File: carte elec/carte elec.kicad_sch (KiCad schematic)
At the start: 47 parts, among them J1 SD_Card_Device, J2 Barrel_Jack_Switch, U1 ESP32-S3-UNO, U2 R-78E5.0-1.0

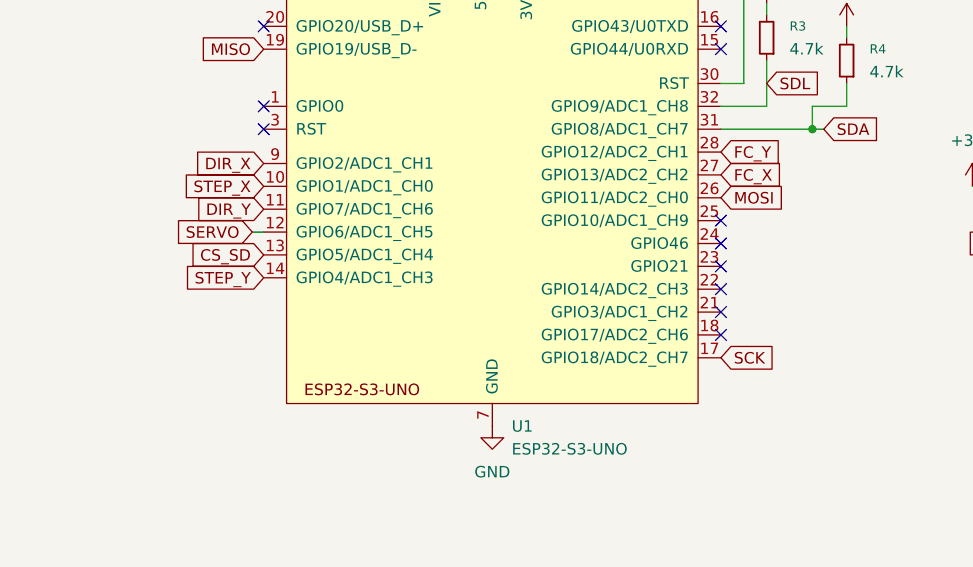
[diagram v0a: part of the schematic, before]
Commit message: Add files via upload
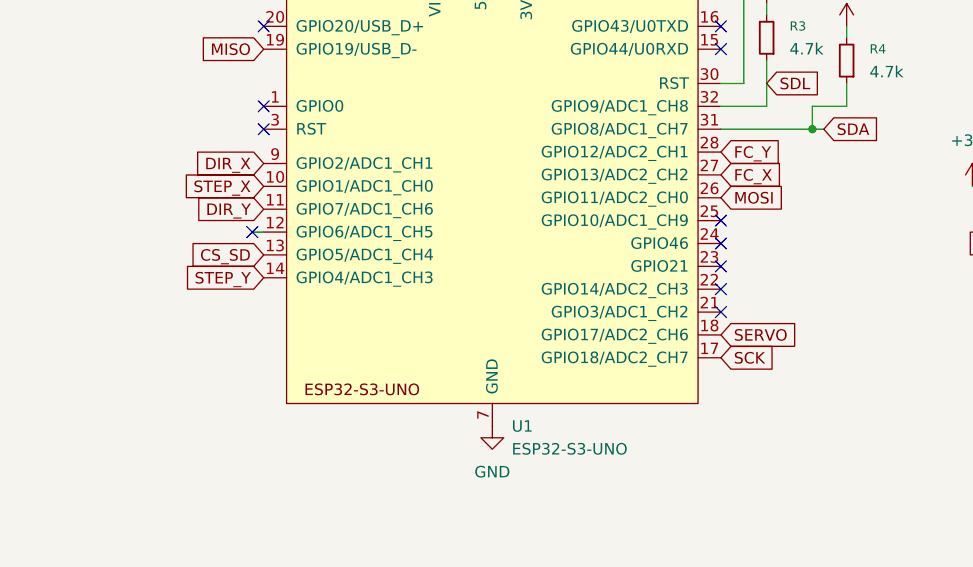
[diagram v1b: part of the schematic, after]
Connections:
- net SERVO: now also U1.18 (GPIO17/ADC2_CH6); no longer U1.12 (GPIO6/ADC1_CH5)
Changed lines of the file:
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@@
+	)
+	(no_connect
+		(at 143.51 129.54)
 	)
 	(no_connect
@@
 	(no_connect
 		(at 248.92 26.67)
-	)
-	(no_connect
-		(at 195.58 140.97)
 	)
 	(no_connect
@@
 		)
 	)
+	(global_label "SERVO"
+		(shape input)
+		(at 195.58 140.97 0)
+		(fields_autoplaced yes)
+		(effects
+			(font
+				(size 1.27 1.27)
+			)
+			(justify left)
+		)
+		(property "Intersheetrefs" "${INTERSHEET_REFS}"
+			(at 204.6128 140.97 0)
+			(effects
+				(font
+					(size 1.27 1.27)
+				)
+				(justify left)
+				(hide yes)
+			)
+		)
+	)
 	(global_label "CS_SD"
 		(shape input)
@@
 			(effects
 				(font
-					(size 1.27 1.27)
-				)
-				(justify right)
-				(hide yes)
-			)
-		)
-	)
-	(global_label "SERVO"
-		(shape input)
-		(at 143.51 129.54 180)
-		(fields_autoplaced yes)
-		(effects
-			(font
-				(size 1.27 1.27)
-			)
-			(justify right)
-		)
-		(property "Intersheetrefs" "${INTERSHEET_REFS}"
-			(at 134.4772 129.54 0)
-			(effects
-				(font

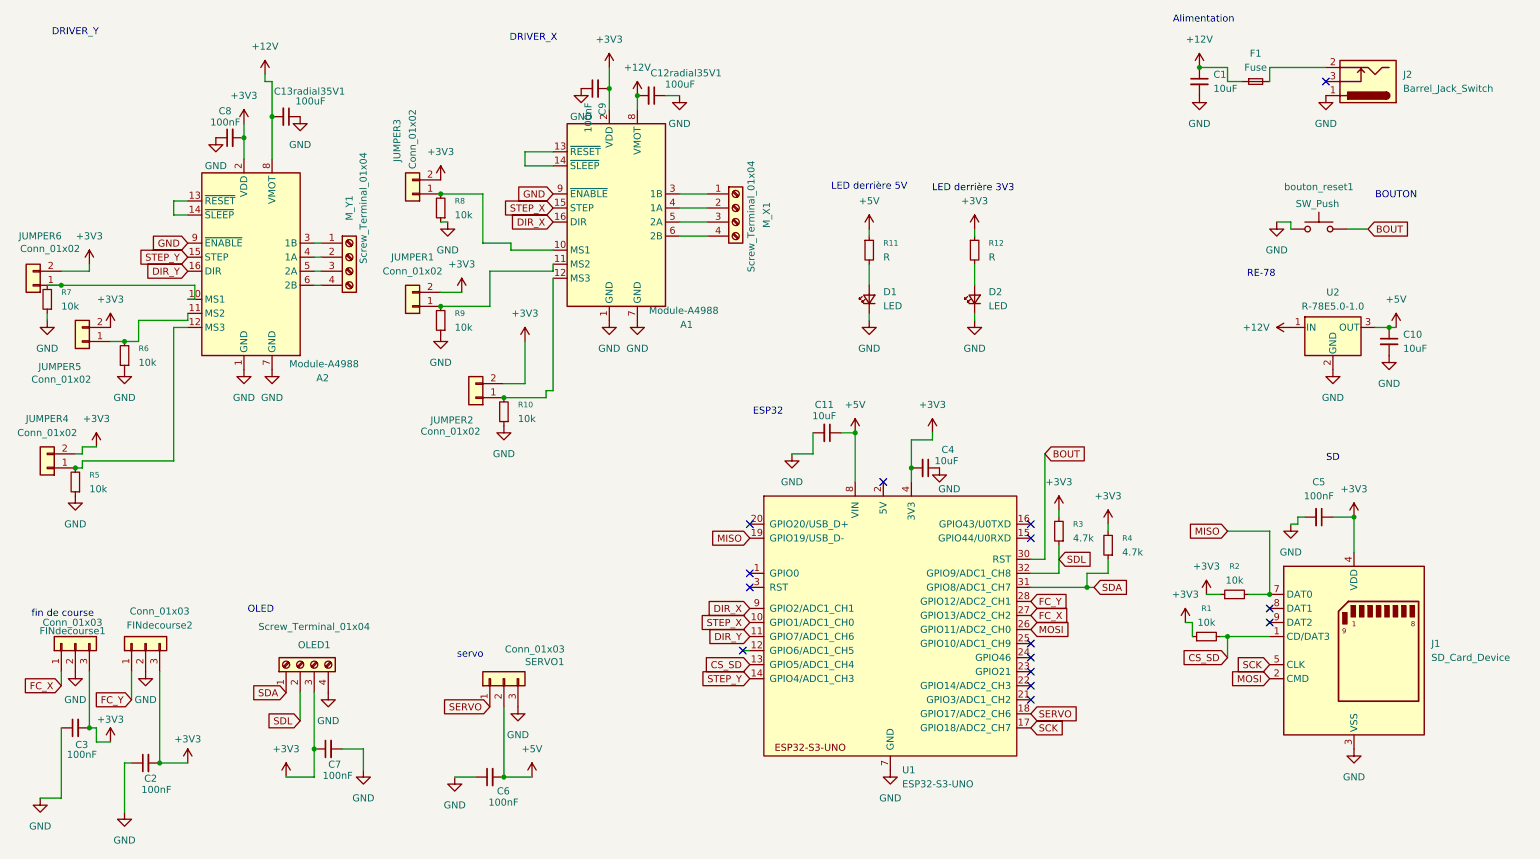
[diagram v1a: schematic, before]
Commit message: Add files via upload
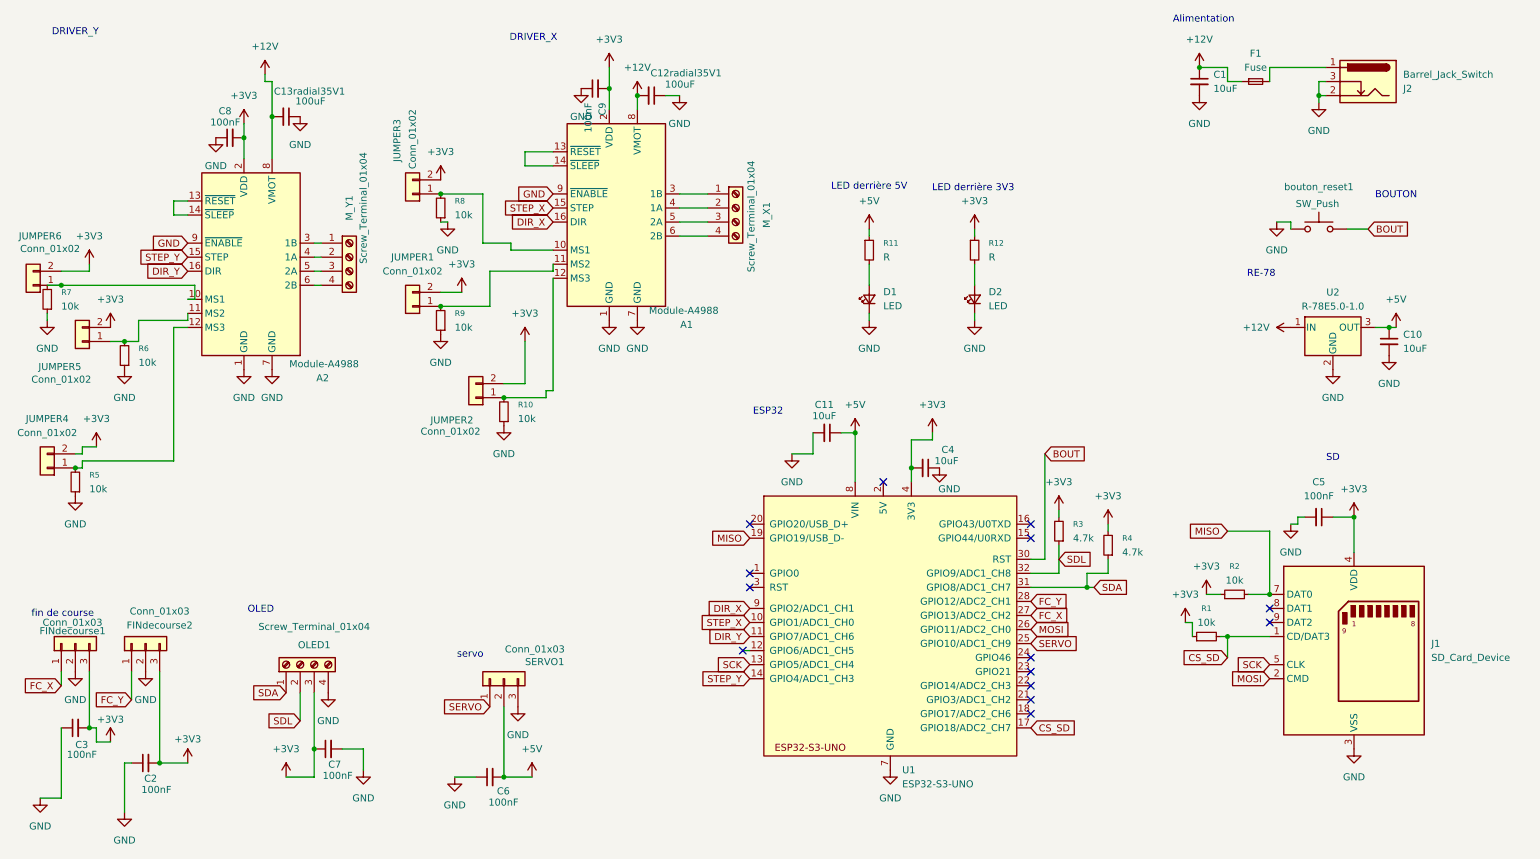
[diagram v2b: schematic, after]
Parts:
- F1: footprint Fuse:Fuse_1206_3216Metric -> Fuse:Fuseholder_Blade_Mini_Keystone_3568
- J2: footprint Connector_BarrelJack:BarrelJack_CUI_PJ-036AH-SMT_Horizontal -> Connector_BarrelJack:BarrelJack_Horizontal
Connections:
- net CS_SD: now also U1.17 (GPIO18/ADC2_CH7); no longer U1.13 (GPIO5/ADC1_CH4)
- net GND: now also J2.2, J2.3; no longer J2.1
- net SCK: now also U1.13 (GPIO5/ADC1_CH4); no longer U1.17 (GPIO18/ADC2_CH7)
- net SERVO: now also U1.25 (GPIO10/ADC1_CH9); no longer U1.18 (GPIO17/ADC2_CH6)
- net at F1.2: now also J2.1; no longer J2.2
- no-connect marks 15 -> 14
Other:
- moved on the sheet: J2
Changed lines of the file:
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@@
 	)
 	(junction
+		(at 247.65 29.21)
+		(diameter 0)
+		(color 0 0 0 0)
+	)
+	(junction
 		(at 163.83 90.17)
 		(diameter 0)
@@
 	)
 	(no_connect
-		(at 143.51 129.54)
+		(at 195.58 140.97)
 	)
 	(no_connect
@@
 	)
 	(no_connect
-		(at 248.92 26.67)
+		(at 143.51 129.54)
 	)
 	(no_connect
@@
 		(at 195.58 109.22)
 	)
-	(no_connect
-		(at 195.58 128.27)
-	)
 	(wire
 		(pts
@@
 	(wire
 		(pts
+			(xy 248.92 26.67) (xy 247.65 26.67)
+		)
+		(stroke
+			(width 0)
+			(type default)
+		)
+	)
+	(wire
+		(pts
 			(xy 104.14 81.28) (xy 100.33 81.28)
 		)
@@
 	(wire
 		(pts
+			(xy 247.65 29.21) (xy 248.92 29.21)
+		)
+		(stroke
+			(width 0)
+			(type default)
+		)
+	)
+	(wire
+		(pts
 			(xy 43.18 50.8) (xy 40.64 50.8)
 		)
@@
 	(wire
 		(pts
+			(xy 247.65 30.48) (xy 247.65 29.21)
+		)
+		(stroke
+			(width 0)
+			(type default)
+		)
+	)
+	(wire
+		(pts
 			(xy 40.64 50.8) (xy 40.64 48.26)
 		)
@@
 	(wire
 		(pts
+			(xy 247.65 26.67) (xy 247.65 29.21)
+		)
+		(stroke
+			(width 0)
+			(type default)
+		)
+	)
+	(wire
+		(pts
 			(xy 152.4 93.98) (xy 156.21 93.98)
 		)
@@
 		)
 	)
+	(global_label "CS_SD"
+		(shape input)
+		(at 195.58 143.51 0)
+		(fields_autoplaced yes)
+		(effects
+			(font
+				(size 1.27 1.27)
+			)
+			(justify left)
+		)
+		(property "Intersheetrefs" "${INTERSHEET_REFS}"
+			(at 204.4918 143.51 0)
+			(effects
+				(font
+					(size 1.27 1.27)
+				)
+				(justify left)
+				(hide yes)
+			)
+		)
+	)
 	(global_label "DIR_X"
 		(shape input)
@@
 		)
 	)
-	(global_label "SERVO"
-		(shape input)
-		(at 195.58 140.97 0)
-		(fields_autoplaced yes)
-		(effects
-			(font
-				(size 1.27 1.27)
-			)
-			(justify left)
-		)
-		(property "Intersheetrefs" "${INTERSHEET_REFS}"
-			(at 204.6128 140.97 0)
-			(effects
-				(font
-					(size 1.27 1.27)
-				)
-				(justify left)
-				(hide yes)
-			)
-		)
-	)
-	(global_label "CS_SD"
-		(shape input)
-		(at 144.78 132.08 180)
-		(fields_autoplaced yes)
-		(effects
-			(font
-				(size 1.27 1.27)
-			)
-			(justify right)
-		)
-		(property "Intersheetrefs" "${INTERSHEET_REFS}"
-			(at 135.8682 132.08 0)
-			(effects
-				(font
-					(size 1.27 1.27)
-				)
-				(justify right)
-				(hide yes)
-			)
-		)
-	)
 	(global_label "MISO"
 		(shape input)
@@
 	(global_label "SCK"
 		(shape input)
-		(at 195.58 143.51 0)
+		(at 144.78 132.08 180)
 		(fields_autoplaced yes)
 		(effects
@@
 				(size 1.27 1.27)
 			)
-			(justify left)
+			(justify right)
 		)
 		(property "Intersheetrefs" "${INTERSHEET_REFS}"
-			(at 202.3147 143.51 0)
+			(at 138.0453 132.08 0)
 			(effects
 				(font
 					(size 1.27 1.27)
 				)
-				(justify left)
+				(justify right)
 				(hide yes)
 			)
@@
 		)
 	)
+	(global_label "SERVO"
+		(shape input)
+		(at 195.58 128.27 0)
+		(fields_autoplaced yes)
+		(effects
+			(font
+				(size 1.27 1.27)
+			)
+			(justify left)
+		)
+		(property "Intersheetrefs" "${INTERSHEET_REFS}"
+			(at 204.6128 128.27 0)
+			(effects
+				(font
+					(size 1.27 1.27)
+				)
+				(justify left)
+				(hide yes)
+			)
+		)
+	)
 	(global_label "SDL"
 		(shape input)
@@
 			)
 		)
-		(property "Footprint" "Fuse:Fuse_1206_3216Metric"
+		(property "Footprint" "Fuse:Fuseholder_Blade_Mini_Keystone_3568"
 			(at 236.22 26.67 0)
 			(effects
@@
 	(symbol
 		(lib_id "power:GND")
-		(at 248.92 29.21 0)
+		(at 247.65 30.48 0)
 		(unit 1)
 		(exclude_from_sim no)
@@
 		(fields_autoplaced yes)
 		(property "Reference" "#PWR033"
-			(at 248.92 35.56 0)
+			(at 247.65 36.83 0)
 			(effects
 				(font
@@
 		)
 		(property "Value" "GND"
-			(at 248.92 34.29 0)
+			(at 247.65 35.56 0)
 			(effects
 				(font
@@
 		)
 		(property "Footprint" ""
-			(at 248.92 29.21 0)
+			(at 247.65 30.48 0)
 			(effects
 				(font
@@
 		)
 		(property "Datasheet" ""
-			(at 248.92 29.21 0)
+			(at 247.65 30.48 0)
 			(effects
 				(font
@@
 		)
 		(property "Description" "Power symbol creates a global label with name \"GND\" , ground"
-			(at 248.92 29.21 0)
+			(at 247.65 30.48 0)
 			(effects
 				(font
@@
 	(symbol
 		(lib_id "makerspace-unilasalle:Barrel_Jack_Switch")
-		(at 256.54 26.67 180)
+		(at 256.54 26.67 0)
+		(mirror y)
 		(unit 1)
 		(exclude_from_sim no)
@@
 		(on_board yes)
 		(dnp no)
-		(fields_autoplaced yes)
 		(property "Reference" "J2"
-			(at 262.89 25.3999 0)
+			(at 262.89 27.9401 0)
 			(effects
 				(font
@@
 		)
 		(property "Value" "Barrel_Jack_Switch"
-			(at 262.89 27.9399 0)
+			(at 262.89 25.4001 0)
 			(effects
 				(font
@@
 			)
 		)
-		(property "Footprint" "Connector_BarrelJack:BarrelJack_CUI_PJ-036AH-SMT_Horizontal"
-			(at 255.27 25.654 0)
+		(property "Footprint" "Connector_BarrelJack:BarrelJack_Horizontal"
+			(at 255.27 27.686 0)
 			(effects
 				(font
@@
 		)
 		(property "Datasheet" "~"
-			(at 255.27 25.654 0)
+			(at 255.27 27.686 0)
 			(effects
 				(font
